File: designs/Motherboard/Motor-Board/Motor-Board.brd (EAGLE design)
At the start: 39 x 100 mm, 71 parts, among them IC1 DRV8814, IC2 DRV8814, IC3 PIC24FJ64GA004, J1 22-05-7028-02, J13 22-05-7048-04, J2 22-05-7028-02, J3 22-05-7048-04, J7 22-05-7028-02, J8 22-05-7028-02, U1 DRV8811PWP, U2 DRV8811PWP

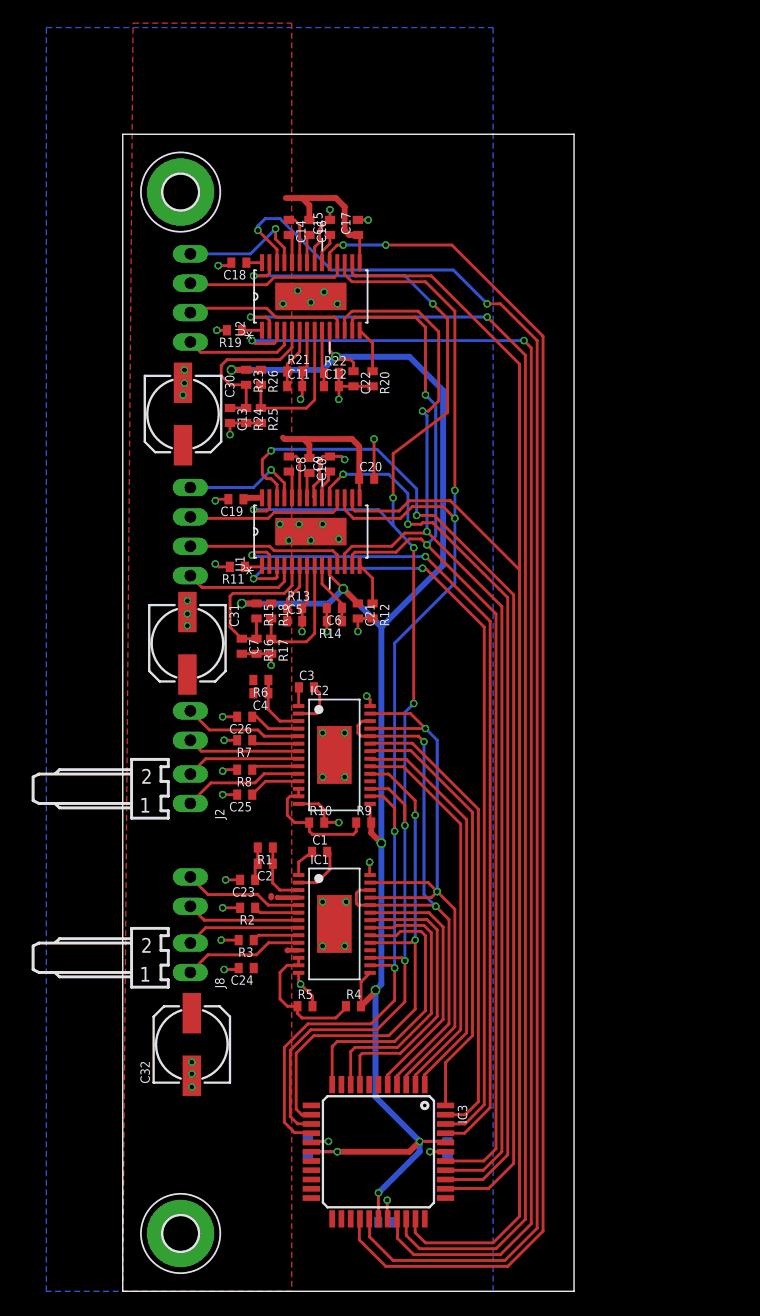
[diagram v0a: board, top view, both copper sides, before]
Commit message: Done with left side of mother board
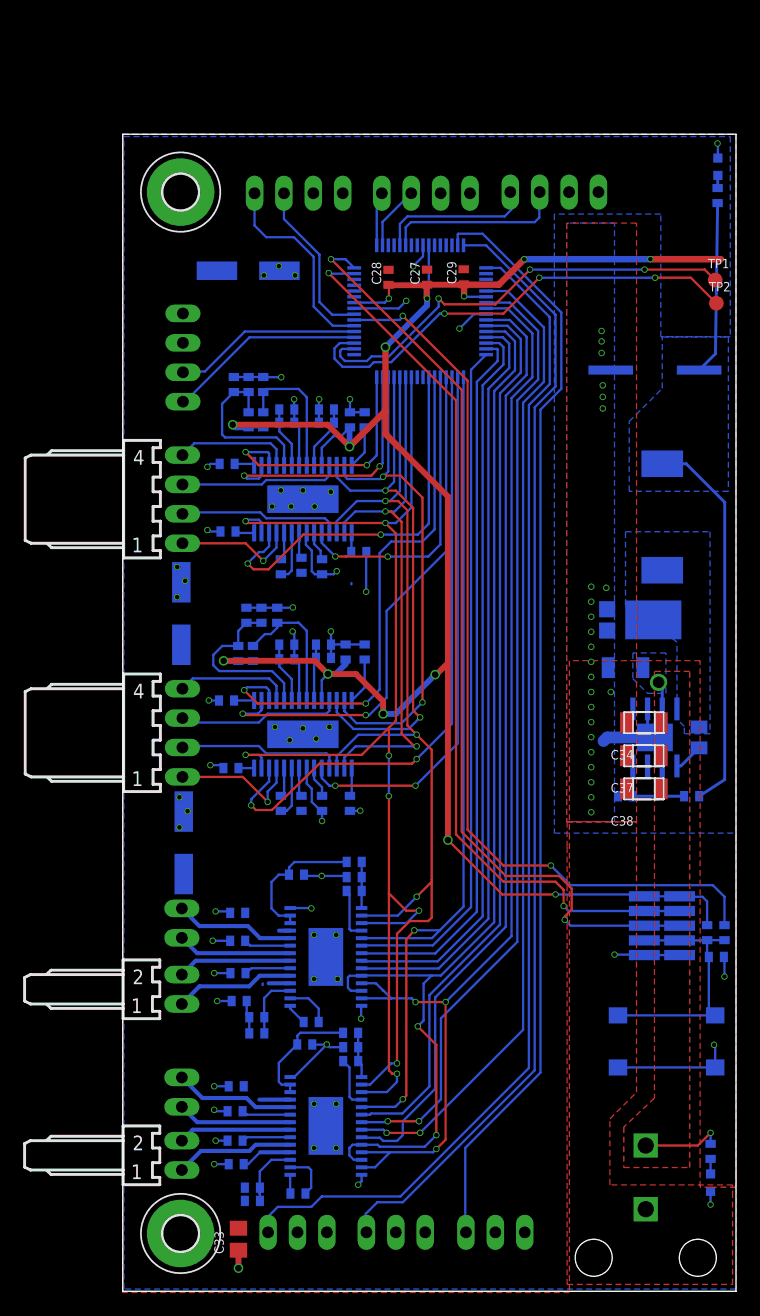
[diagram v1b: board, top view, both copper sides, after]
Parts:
- removed IC3: PIC24FJ64GA004, microchip:TQFP44
- removed J1, J2, J7, J8: 22-05-7028-02, Son_of_Dark_Power:7395-02
- removed J13, J3: 22-05-7048-04, Son_of_Dark_Power:7395-04
- added C33: 10uF, rcl:C0805
- added C34, C37, C38, C39: 4.7uF, 5v:1206
- added C35: 10nF, 5v:0805
- added C36: 330uF, 5v:SM_RADIAL_10AMM
- added C40: .1uF, rcl:C0402
- added C41, C42: 0.47uF, rcl:C0402
- added D2: PDS760-13, 5v:POWERDI5
- added IC4: PIC24FJ256GB106, microchip:TQFP64-10X10
- added L1: (no value), WE-HCC:WE-HCC_1090
- added LED4, POWER_ON: (no value), led:CHIP-LED0603
- added MOTIN1, MOTIN2, MOTIN3, MOTIN4, STEP1, STEP2: 22-05-7048-04, Son_of_Dark_Power:7395-04
- added MOTOR1, MOTOR2, MOTOR3, MOTOR4: 22-05-7028-02, Son_of_Dark_Power:7395-02
- added PROGRAMMING: Jtag, Mother-Board-rev5:MOTHER-BOARD-REV5_10-PIN-SMD
- added PWR_IN(2): (no value), Son_of_Dark_Powersch:5569-2
- added R27, R29, R31, R32, R33, R34: 10k, rcl:R0402
- added R28: (no value), rcl:R0402
- added R30: 100, rcl:R0402
- added SERVO_1, SERVO_2, SERVO_3: (no value), con-molex:7395-03
- added TP1, TP2: PTR1B1,27, testpad:B1,27
- added U$2: TPS5450DDAR, 5v:R-PDSO-G8
- added U$5: Switch3, Parts4Class:MC32882_FINAL
- C1, C23, C24, C25, C26, C3: value (none) -> 0.01uF
- C10, C14, C15, C16, C8, C9: value (none) -> 0.22uF
- C11, C12, C5, C6: value (none) -> 1nF
- C13: value (none) -> .1uF
- C17, C18, C19, C2, C20, C21, C22, C28, C29, C4, C7: value (none) -> 0.1uF
- C27: value (none) -> 1uF
- R1, R6: value (none) -> 1M
- R10, R5: value (none) -> 30k
- R11, R12, R19, R20: value (none) -> 0.1
- R13, R14, R21, R22: value (none) -> 47k
- R15, R16, R17, R18, R23, R24, R25, R26, R4, R9: value (none) -> 10k
- R2, R3, R7, R8: value (none) -> 0.2
- moved C28 81.7 mm to (23.0, 87.6), flipped to the top, turned to 90 degrees
- moved C27 75.9 mm to (26.3, 87.6), flipped to the top
- moved C29 75.4 mm to (29.5, 87.7), flipped to the top, turned to 90 degrees
- moved C14 49.8 mm to (13.7, 42.2), flipped to the bottom, turned to 90 degrees
- moved C15 49.8 mm to (17.2, 42.2), flipped to the bottom, turned to 270 degrees
- moved C16 49.8 mm to (15.4, 42.2), flipped to the bottom, turned to 90 degrees
- moved C17 49.8 mm to (19.6, 42.2), flipped to the bottom, turned to 270 degrees
- moved R6 45.0 mm to (11.2, 7.82), flipped to the bottom, turned to 0 degrees
- moved C3 43.8 mm to (15.1, 8.45), flipped to the bottom, turned to 180 degrees
- moved C18 43.7 mm to (9.35, 45.2), flipped to the bottom, turned to 0 degrees
- moved C4 42.7 mm to (11.2, 8.96), flipped to the bottom, turned to 0 degrees
- moved C26 38.7 mm to (9.81, 11.0), flipped to the bottom, turned to 0 degrees
- moved U2 37.8 mm to (15.6, 48.1), flipped to the bottom, turned to 270 degrees
- moved R7 34.6 mm to (9.71, 13.0), flipped to the bottom, turned to 0 degrees
- moved C31 32.6 mm to (10.8, 88.2), flipped to the bottom, turned to 0 degrees
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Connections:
- removed net M1-NFAULT: IC1.18
- removed net M2-NFAULT: IC2.18
- removed net MCLR: IC3.18
- removed net PGC1: IC3.22
- removed net PGD1: IC3.21
- new net AVDD: IC4.19
- new net AVSS: IC4.20
- new net BOOT_VM: C35.1, U$2.1
- new net CHANNEL_A_1: IC4.4, MOTIN1.4
- new net CHANNEL_A_2: IC4.22, MOTIN2.3
- new net CHANNEL_A_3: IC4.18, MOTIN3.3
- new net CHANNEL_A_4: IC4.8, MOTIN4.3
- new net CHANNEL_B_1: IC4.5, MOTIN1.3
- new net CHANNEL_B_2: IC4.21, MOTIN2.4
- new net CHANNEL_B_3: IC4.17, MOTIN3.4
- new net CHANNEL_B_4: IC4.6, MOTIN4.4
- new net M_MCLR: C40.1, PROGRAMMING.7, PROGRAMMING.8, R30.2, R31.1, U$5.P$2, U$5.P$3
- new net M_MCLR': IC4.7, R30.1
- new net M_PGC1: IC4.15, PROGRAMMING.3, PROGRAMMING.4
- new net M_PGD1: IC4.16, PROGRAMMING.5, PROGRAMMING.6
- new net N$25: LED4.A, R29.1
- new net N$29: C41.1, IC1.15, R32.2, R4.2
- new net N$31: IC1.18, R32.1
- new net N$35: IC2.18, R33.1
- new net N$37: C42.1, IC2.15, R33.2, R9.2
- new net N$38: POWER_ON.A, R34.1
- new net OC1: IC4.33, SERVO_1.1
- new net OC2: IC4.32, SERVO_2.1
- new net OC3: IC4.31, SERVO_3.1
- new net PH_VM: C35.2, D2.3, L1.1, U$2.8
- new net VCC: C34.2, C37.2, C38.2, C39.2, PWR_IN(2).2, R34.2, U$2.7
- new net VSNS_VM: R27.1, R28.2, U$2.4
- net +3V3: now also IC4.10, IC4.26, IC4.38, PROGRAMMING.1, PROGRAMMING.2, R31.2; no longer IC1.15, IC2.15, IC3.17, IC3.28, IC3.40, R4.2, R9.2
- net +7V: now also C33.1, C36.1, H2.B3,0, L1.2, MOTIN1.2, MOTIN2.2, MOTIN3.2, MOTIN4.2, R27.2, R29.2, SERVO_1.2, SERVO_2.2, SERVO_3.2
- net GND: now also C33.2, C34.1, C36.2, C37.1, C38.1, C39.1, C40.2, C41.2, C42.2, D2.1, IC4.25, IC4.41, IC4.9, LED4.C, MOTIN1.1, MOTIN2.1, MOTIN3.1, MOTIN4.1, POWER_ON.C, PROGRAMMING.10, PROGRAMMING.9, PWR_IN(2).1, R28.1, SERVO_1.3, SERVO_2.3, SERVO_3.3, U$2.6, U$2.9, U$5.P$1, U$5.P$4; no longer IC3.16, IC3.29, IC3.39
- net M-DECAY: now also IC4.49; no longer IC3.13
- net M-I0: now also IC4.44; no longer IC3.4
- net M-I1: now also IC4.40; no longer IC3.3
- net M-NSLEEP: now also IC4.58; no longer IC3.14
- net M-RESET: now also IC4.60; no longer IC3.15
- net M1-AENBL: now also IC4.47; no longer IC3.9
- net M1-APHASE: now also IC4.48; no longer IC3.11
- net M1-BENBL: now also IC4.46; no longer IC3.8
- net M1-BHPASE: now also IC4.45; no longer IC3.5
- net M1-MAOUT1: now also MOTOR2.1; no longer J7.1
- net M1-MAOUT2: now also MOTOR2.2; no longer J7.2
- net M1-MBOUT1: now also MOTOR1.1; no longer J8.1
- net M1-MBOUT2: now also MOTOR1.2; no longer J8.2
- net M2-AENBL: now also IC4.39; no longer IC3.1
- net M2-APHASE: now also IC4.43; no longer IC3.2
- net M2-BENBL: now also IC4.37; no longer IC3.44
- net M2-BHPASE: now also IC4.42; no longer IC3.43
- net M2-MAOUT1: now also MOTOR4.1; no longer J1.1
- net M2-MAOUT2: now also MOTOR4.2; no longer J1.2
- net M2-MBOUT1: now also MOTOR3.1; no longer J2.1
- net M2-MBOUT2: now also MOTOR3.2; no longer J2.2
- net S-SRN: now also IC4.59; no longer IC3.32
- net S1-AOUT1: now also STEP1.4; no longer J3.4
- net S1-AOUT2: now also STEP1.1; no longer J3.1
- net S1-BOUT1: now also STEP1.3; no longer J3.3
- net S1-BOUT2: now also STEP1.2; no longer J3.2
- net S1-DIR: now also IC4.64; no longer IC3.42
- net S1-ENABLEN: now also IC4.55; no longer IC3.35
- net S1-HOME: now also IC4.63; no longer IC3.41
- net S1-STEP: now also IC4.53; no longer IC3.36
- net S2-AOUT1: now also STEP2.4; no longer J13.4
- net S2-AOUT2: now also STEP2.1; no longer J13.1
- net S2-BOUT1: now also STEP2.3; no longer J13.3
- net S2-BOUT2: now also STEP2.2; no longer J13.2
- net S2-DIR: now also IC4.54; no longer IC3.30
- net S2-ENABLEN: now also IC4.51; no longer IC3.27
- net S2-HOME: now also IC4.52; no longer IC3.31
- net S2-STEP: now also IC4.50; no longer IC3.26
- net SCL: now also IC4.2, TP1.TP; no longer IC3.24
- net SDA: now also IC4.3, TP2.TP; no longer IC3.23
- net USM0: now also IC4.62; no longer IC3.38
- net USM1: now also IC4.61; no longer IC3.37
- net VDDCORE: now also IC4.56; no longer IC3.7
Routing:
- net OC1: track 0.00 -> 102.2 mm
- net OC2: track 0.00 -> 97.8 mm
- net OC3: track 0.00 -> 95.7 mm
- net M_PGD1: track 0.00 -> 81.1 mm, vias 0 -> 2
- net M_PGC1: track 0.00 -> 78.2 mm, vias 0 -> 2
- net M_MCLR': track 0.00 -> 78.2 mm, vias 0 -> 2
- net S-SRN: track 122.1 -> 47.0 mm, vias 0 -> 2
- net S2-STEP: track 120.1 -> 46.1 mm
- net S2-ENABLEN: track 127.4 -> 54.4 mm
- net S2-DIR: track 118.3 -> 46.5 mm
- net S2-HOME: track 115.7 -> 45.6 mm
- net S1-ENABLEN: track 88.6 -> 33.8 mm
- net USM1: track 99.2 -> 46.4 mm
- net USM0: track 94.8 -> 44.0 mm
- net S1-STEP: track 77.2 -> 26.5 mm
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- added copper zone on layer 16, net +7V
- added copper zone on layer 1, net GND
- added copper zone on layer 16, net PH_VM
- added copper zone on layer 1, net VCC
- added copper zone on layer 16, net VCC
- removed copper zone on layer 1, net +7V
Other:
- board size 39 x 100 mm -> 53 x 100 mm
